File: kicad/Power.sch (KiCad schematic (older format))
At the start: 19 parts, among them U201 TPS54232, U202 TC1262-33

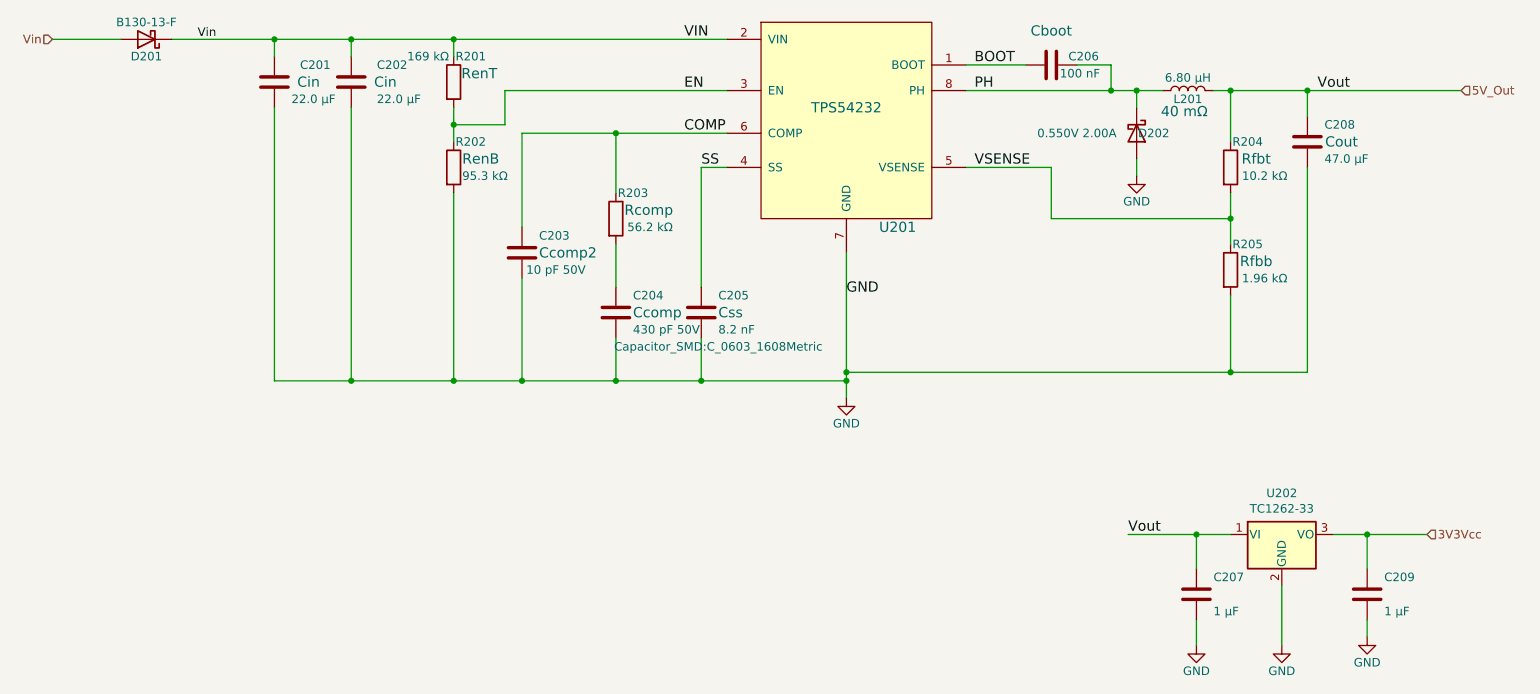
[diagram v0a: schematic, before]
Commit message: Updated the addresssing of the LCD
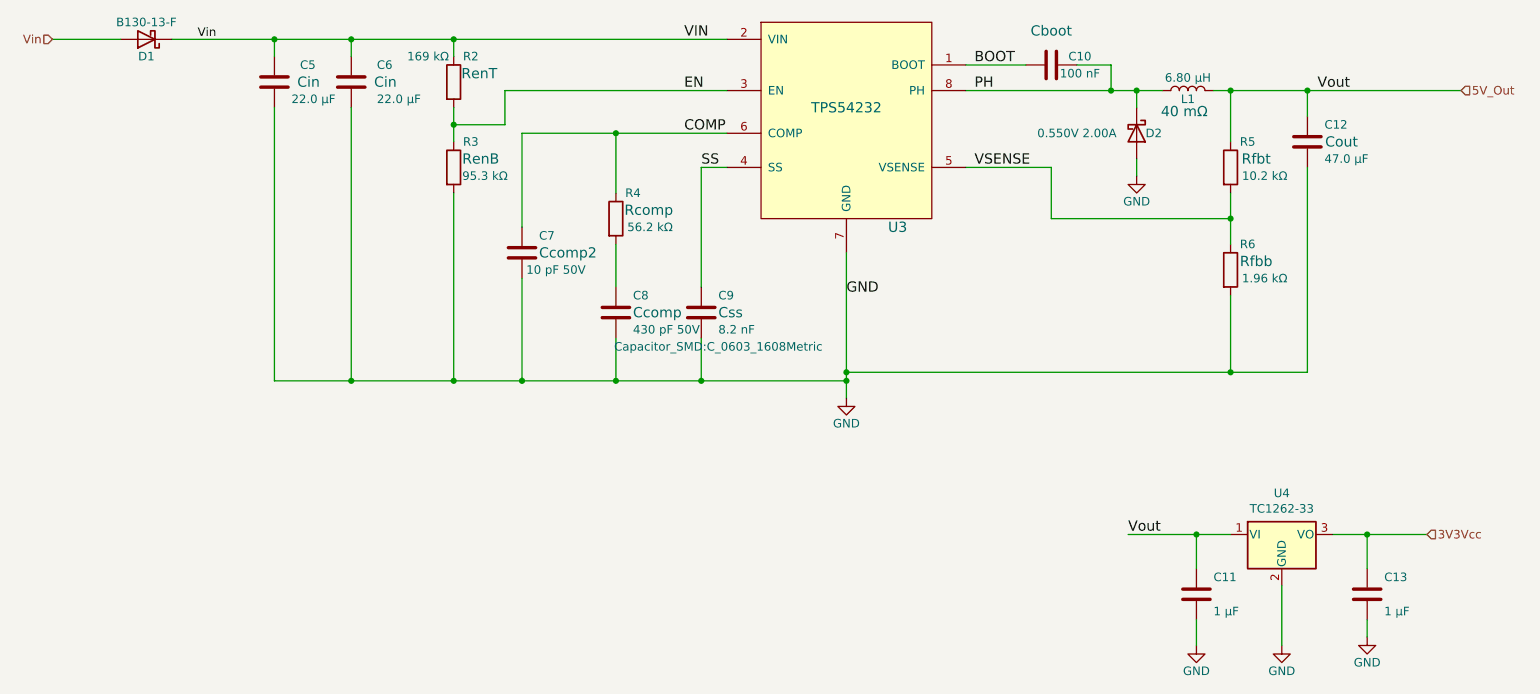
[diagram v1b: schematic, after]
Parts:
- renumbered C206 to C10, C207 to C11, C208 to C12, C209 to C13, C201 to C5, C202 to C6, C203 to C7, C204 to C8, C205 to C9, D201 to D1, D202 to D2, L201 to L1, R201 to R2, R202 to R3, R203 to R4, R204 to R5, R205 to R6, U201 to U3, U202 to U4
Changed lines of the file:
@@
 $EndDescr
 $Comp
-L FieldDevice_Power_5V-rescue:TPS54232-FieldDevice_Power_5V U201
+L FieldDevice_Power_5V-rescue:TPS54232-FieldDevice_Power_5V U3
 U 1 1 5A47974C
 P 5600 1700
-F 0 "U201" H 5900 1000 60  0000 C CNN
+F 0 "U3" H 5900 1000 60  0000 C CNN
 F 1 "TPS54232" H 5600 1700 60  0000 C CNN
 F 2 "FieldDevice_Power_5V:TPS54232DR" H 5600 1750 60  0001 C CNN
@@
 $EndComp
 $Comp
-L Device:R R201
+L Device:R R2
 U 1 1 5A47979B
 P 3300 1550
-F 0 "R201" H 3400 1700 50  0000 C CNN
+F 0 "R2" H 3400 1700 50  0000 C CNN
 F 1 "169 kΩ" H 3150 1700 50  0000 C CNN
 F 2 "Resistor_SMD:R_0805_2012Metric" V 3230 1550 50  0001 C CNN
@@
 $EndComp
 $Comp
-L Device:R R202
+L Device:R R3
 U 1 1 5A47981A
 P 3300 2050
-F 0 "R202" H 3400 2200 50  0000 C CNN
+F 0 "R3" H 3400 2200 50  0000 C CNN
 F 1 "95.3 kΩ" H 3350 2000 50  0000 L CNN
 F 2 "Resistor_SMD:R_0805_2012Metric" V 3230 2050 50  0001 C CNN
@@
 $EndComp
 $Comp
-L Device:R R203
+L Device:R R4
 U 1 1 5A47984F
 P 4250 2350
-F 0 "R203" H 4350 2500 50  0000 C CNN
+F 0 "R4" H 4350 2500 50  0000 C CNN
 F 1 "56.2 kΩ" H 4450 2300 50  0000 C CNN
 F 2 "Resistor_SMD:R_0805_2012Metric" V 4180 2350 50  0001 C CNN
@@
 $EndComp
 $Comp
-L Device:R R204
+L Device:R R5
 U 1 1 5A479895
 P 7850 2050
-F 0 "R204" H 7950 2200 50  0000 C CNN
+F 0 "R5" H 7950 2200 50  0000 C CNN
 F 1 "10.2 kΩ" H 8050 2000 50  0000 C CNN
 F 2 "Resistor_SMD:R_0805_2012Metric" V 7780 2050 50  0001 C CNN
@@
 $EndComp
 $Comp
-L Device:R R205
+L Device:R R6
 U 1 1 5A479906
 P 7850 2650
-F 0 "R205" H 7950 2800 50  0000 C CNN
+F 0 "R6" H 7950 2800 50  0000 C CNN
 F 1 "1.96 kΩ" H 8050 2600 50  0000 C CNN
 F 2 "Resistor_SMD:R_0805_2012Metric" V 7780 2650 50  0001 C CNN
@@
 $EndComp
 $Comp
-L Device:C C201
+L Device:C C5
 U 1 1 5A479940
 P 2250 1550
-F 0 "C201" H 2400 1650 50  0000 L CNN
+F 0 "C5" H 2400 1650 50  0000 L CNN
 F 1 "22.0 μF" H 2350 1450 50  0000 L CNN
 F 2 "Capacitor_SMD:C_1210_3225Metric" H 2100 1450 50  0001 C CNN
@@
 $EndComp
 $Comp
-L Device:C C203
+L Device:C C7
 U 1 1 5A4799E0
 P 3700 2550
-F 0 "C203" H 3800 2650 50  0000 L CNN
+F 0 "C7" H 3800 2650 50  0000 L CNN
 F 1 "10 pF 50V" H 3725 2450 50  0000 L CNN
 F 2 "Capacitor_SMD:C_0805_2012Metric" H 3738 2400 50  0001 C CNN
@@
 $EndComp
 $Comp
-L Device:C C204
+L Device:C C8
 U 1 1 5A479A24
 P 4250 2900
-F 0 "C204" H 4350 3000 50  0000 L CNN
+F 0 "C8" H 4350 3000 50  0000 L CNN
 F 1 "430 pF 50V" H 4350 2800 50  0000 L CNN
 F 2 "Capacitor_SMD:C_0805_2012Metric" H 4288 2750 50  0001 C CNN
@@
 $EndComp
 $Comp
-L Device:C C205
+L Device:C C9
 U 1 1 5A479A65
 P 4750 2900
-F 0 "C205" H 4850 3000 50  0000 L CNN
+F 0 "C9" H 4850 3000 50  0000 L CNN
 F 1 "8.2 nF" H 4850 2800 50  0000 L CNN
 F 2 "Capacitor_SMD:C_0603_1608Metric" H 4850 2700 50  0000 C CNN
@@
 $EndComp
 $Comp
-L Device:C C206
+L Device:C C10
 U 1 1 5A479AA7
 P 6800 1450
-F 0 "C206" V 6750 1550 50  0000 L CNN
+F 0 "C10" V 6750 1550 50  0000 L CNN
 F 1 "100 nF" V 6850 1500 50  0000 L CNN
 F 2 "Capacitor_SMD:C_0805_2012Metric" H 6838 1300 50  0001 C CNN
@@
 $EndComp
 $Comp
-L Device:C C208
+L Device:C C12
 U 1 1 5A479B0E
 P 8300 1900
-F 0 "C208" H 8400 2000 50  0000 L CNN
+F 0 "C12" H 8400 2000 50  0000 L CNN
 F 1 "47.0 μF" H 8400 1800 50  0000 L CNN
 F 2 "Capacitor_SMD:C_0805_2012Metric" H 8338 1750 50  0001 C CNN
@@
 $EndComp
 $Comp
-L Device:L L201
+L Device:L L1
 U 1 1 5A479B7A
 P 7600 1600
-F 0 "L201" V 7550 1600 50  0000 C CNN
+F 0 "L1" V 7550 1600 50  0000 C CNN
 F 1 "6.80 μΗ" V 7675 1600 50  0000 C CNN
 F 2 "FieldDevice_Power_5V:SDR0805-6R8ML" H 7600 1600 50  0001 C CNN
@@
 $EndComp
 $Comp
-L Device:D_Schottky D202
+L Device:D_Schottky D2
 U 1 1 5A479CF1
 P 7300 1850
-F 0 "D202" V 7300 1950 50  0000 C CNN
+F 0 "D2" V 7300 1950 50  0000 C CNN
 F 1 "0.550V 2.00A" V 7300 1500 50  0000 C CNN
 F 2 "FieldDevice_Power_5V:D_SOD-123F" H 7300 1850 50  0001 C CNN
@@
 $EndComp
 $Comp
-L Device:C C202
+L Device:C C6
 U 1 1 5A47A146
 P 2700 1550
-F 0 "C202" H 2850 1650 50  0000 L CNN
+F 0 "C6" H 2850 1650 50  0000 L CNN
 F 1 "22.0 μF" H 2850 1450 50  0000 L CNN
 F 2 "Capacitor_SMD:C_1210_3225Metric" H 2600 1650 50  0001 C CNN
@@
 	3300 1700 3300 1800
 $Comp
-L power:GND #PWR0201
+L power:GND #PWR011
 U 1 1 5A47B13B
 P 5600 3400
-F 0 "#PWR0201" H 5600 3150 50  0001 C CNN
+F 0 "#PWR011" H 5600 3150 50  0001 C CNN
 F 1 "GND" H 5600 3250 50  0000 C CNN
 F 2 "" H 5600 3400 50  0001 C CNN
@@
 $EndComp
 $Comp
-L power:GND #PWR0202
+L power:GND #PWR012
 U 1 1 5A47B17A
 P 7300 2100
-F 0 "#PWR0202" H 7300 1850 50  0001 C CNN
+F 0 "#PWR012" H 7300 1850 50  0001 C CNN
 F 1 "GND" H 7300 1950 50  0000 C CNN
 F 2 "" H 7300 2100 50  0001 C CNN
@@
 Vout
 $Comp
-L Device:D_Schottky D201
+L Device:D_Schottky D1
 U 1 1 5A482394
 P 1500 1300
-F 0 "D201" H 1500 1400 50  0000 C CNN
+F 0 "D1" H 1500 1400 50  0000 C CNN
 F 1 "B130-13-F" H 1500 1200 50  0000 C CNN
 F 2 "FieldDevice_Power_5V:B130-13-F" H 1500 1300 50  0001 C CNN
@@
 5V_Out
 $Comp
-L Regulator_Linear:TC1262-33 U202
+L Regulator_Linear:TC1262-33 U4
 U 1 1 5F29C039
 P 8150 4200
-F 0 "U202" H 8150 4442 50  0000 C CNN
+F 0 "U4" H 8150 4442 50  0000 C CNN
 F 1 "TC1262-33" H 8150 4351 50  0000 C CNN
 F 2 "" H 8150 4425 50  0001 C CIN
@@
 	8150 4500 8150 4850
 $Comp
-L power:GND #PWR0204
+L power:GND #PWR014
 U 1 1 5F2AC1B9
 P 8150 4850
-F 0 "#PWR0204" H 8150 4600 50  0001 C CNN
+F 0 "#PWR014" H 8150 4600 50  0001 C CNN
 F 1 "GND" H 8150 4700 50  0000 C CNN
 F 2 "" H 8150 4850 50  0001 C CNN
@@
 $EndComp
 $Comp
-L Device:C C207
+L Device:C C11
 U 1 1 5F2ACA63
 P 7650 4550
-F 0 "C207" H 7750 4650 50  0000 L CNN
+F 0 "C11" H 7750 4650 50  0000 L CNN
 F 1 "1 μF" H 7750 4450 50  0000 L CNN
 F 2 "Capacitor_SMD:C_0805_2012Metric" H 7688 4400 50  0001 C CNN
@@
 	8650 4200 9000 4200
 $Comp
-L power:GND #PWR0203
+L power:GND #PWR013
 U 1 1 5F2AE872
 P 7650 4850
-F 0 "#PWR0203" H 7650 4600 50  0001 C CNN
+F 0 "#PWR013" H 7650 4600 50  0001 C CNN
 F 1 "GND" H 7650 4700 50  0000 C CNN
 F 2 "" H 7650 4850 50  0001 C CNN
@@
 	7650 4200 7250 4200
 $Comp
-L Device:C C209
+L Device:C C13
 U 1 1 5F2B414B
 P 8650 4550
-F 0 "C209" H 8750 4650 50  0000 L CNN
+F 0 "C13" H 8750 4650 50  0000 L CNN
 F 1 "1 μF" H 8750 4450 50  0000 L CNN
 F 2 "Capacitor_SMD:C_0805_2012Metric" H 8688 4400 50  0001 C CNN
@@
 $EndComp
 $Comp
-L power:GND #PWR0205
+L power:GND #PWR015
 U 1 1 5F2B4985
 P 8650 4800
-F 0 "#PWR0205" H 8650 4550 50  0001 C CNN
+F 0 "#PWR015" H 8650 4550 50  0001 C CNN
 F 1 "GND" H 8650 4650 50  0000 C CNN
 F 2 "" H 8650 4800 50  0001 C CNN

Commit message: Updates the RC selection for the switch debounce
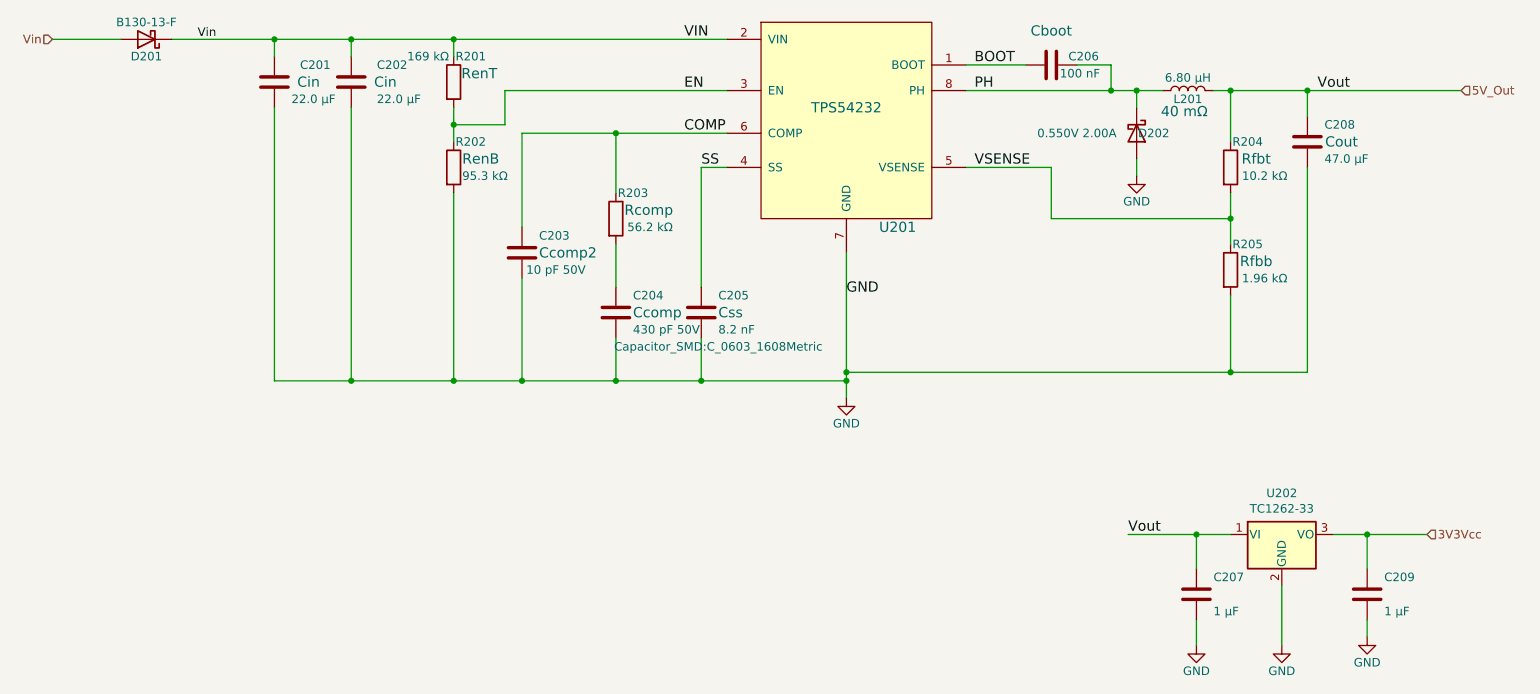
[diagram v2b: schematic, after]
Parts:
- renumbered C5 to C201, C6 to C202, C7 to C203, C8 to C204, C9 to C205, C10 to C206, C11 to C207, C12 to C208, C13 to C209, D1 to D201, D2 to D202, L1 to L201, R2 to R201, R3 to R202, R4 to R203, R5 to R204, R6 to R205, U3 to U201, U4 to U202
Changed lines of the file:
@@
 $EndDescr
 $Comp
-L FieldDevice_Power_5V-rescue:TPS54232-FieldDevice_Power_5V U3
+L FieldDevice_Power_5V-rescue:TPS54232-FieldDevice_Power_5V U201
 U 1 1 5A47974C
 P 5600 1700
-F 0 "U3" H 5900 1000 60  0000 C CNN
+F 0 "U201" H 5900 1000 60  0000 C CNN
 F 1 "TPS54232" H 5600 1700 60  0000 C CNN
 F 2 "FieldDevice_Power_5V:TPS54232DR" H 5600 1750 60  0001 C CNN
@@
 $EndComp
 $Comp
-L Device:R R2
+L Device:R R201
 U 1 1 5A47979B
 P 3300 1550
-F 0 "R2" H 3400 1700 50  0000 C CNN
+F 0 "R201" H 3400 1700 50  0000 C CNN
 F 1 "169 kΩ" H 3150 1700 50  0000 C CNN
 F 2 "Resistor_SMD:R_0805_2012Metric" V 3230 1550 50  0001 C CNN
@@
 $EndComp
 $Comp
-L Device:R R3
+L Device:R R202
 U 1 1 5A47981A
 P 3300 2050
-F 0 "R3" H 3400 2200 50  0000 C CNN
+F 0 "R202" H 3400 2200 50  0000 C CNN
 F 1 "95.3 kΩ" H 3350 2000 50  0000 L CNN
 F 2 "Resistor_SMD:R_0805_2012Metric" V 3230 2050 50  0001 C CNN
@@
 $EndComp
 $Comp
-L Device:R R4
+L Device:R R203
 U 1 1 5A47984F
 P 4250 2350
-F 0 "R4" H 4350 2500 50  0000 C CNN
+F 0 "R203" H 4350 2500 50  0000 C CNN
 F 1 "56.2 kΩ" H 4450 2300 50  0000 C CNN
 F 2 "Resistor_SMD:R_0805_2012Metric" V 4180 2350 50  0001 C CNN
@@
 $EndComp
 $Comp
-L Device:R R5
+L Device:R R204
 U 1 1 5A479895
 P 7850 2050
-F 0 "R5" H 7950 2200 50  0000 C CNN
+F 0 "R204" H 7950 2200 50  0000 C CNN
 F 1 "10.2 kΩ" H 8050 2000 50  0000 C CNN
 F 2 "Resistor_SMD:R_0805_2012Metric" V 7780 2050 50  0001 C CNN
@@
 $EndComp
 $Comp
-L Device:R R6
+L Device:R R205
 U 1 1 5A479906
 P 7850 2650
-F 0 "R6" H 7950 2800 50  0000 C CNN
+F 0 "R205" H 7950 2800 50  0000 C CNN
 F 1 "1.96 kΩ" H 8050 2600 50  0000 C CNN
 F 2 "Resistor_SMD:R_0805_2012Metric" V 7780 2650 50  0001 C CNN
@@
 $EndComp
 $Comp
-L Device:C C5
+L Device:C C201
 U 1 1 5A479940
 P 2250 1550
-F 0 "C5" H 2400 1650 50  0000 L CNN
+F 0 "C201" H 2400 1650 50  0000 L CNN
 F 1 "22.0 μF" H 2350 1450 50  0000 L CNN
 F 2 "Capacitor_SMD:C_1210_3225Metric" H 2100 1450 50  0001 C CNN
@@
 $EndComp
 $Comp
-L Device:C C7
+L Device:C C203
 U 1 1 5A4799E0
 P 3700 2550
-F 0 "C7" H 3800 2650 50  0000 L CNN
+F 0 "C203" H 3800 2650 50  0000 L CNN
 F 1 "10 pF 50V" H 3725 2450 50  0000 L CNN
 F 2 "Capacitor_SMD:C_0805_2012Metric" H 3738 2400 50  0001 C CNN
@@
 $EndComp
 $Comp
-L Device:C C8
+L Device:C C204
 U 1 1 5A479A24
 P 4250 2900
-F 0 "C8" H 4350 3000 50  0000 L CNN
+F 0 "C204" H 4350 3000 50  0000 L CNN
 F 1 "430 pF 50V" H 4350 2800 50  0000 L CNN
 F 2 "Capacitor_SMD:C_0805_2012Metric" H 4288 2750 50  0001 C CNN
@@
 $EndComp
 $Comp
-L Device:C C9
+L Device:C C205
 U 1 1 5A479A65
 P 4750 2900
-F 0 "C9" H 4850 3000 50  0000 L CNN
+F 0 "C205" H 4850 3000 50  0000 L CNN
 F 1 "8.2 nF" H 4850 2800 50  0000 L CNN
 F 2 "Capacitor_SMD:C_0603_1608Metric" H 4850 2700 50  0000 C CNN
@@
 $EndComp
 $Comp
-L Device:C C10
+L Device:C C206
 U 1 1 5A479AA7
 P 6800 1450
-F 0 "C10" V 6750 1550 50  0000 L CNN
+F 0 "C206" V 6750 1550 50  0000 L CNN
 F 1 "100 nF" V 6850 1500 50  0000 L CNN
 F 2 "Capacitor_SMD:C_0805_2012Metric" H 6838 1300 50  0001 C CNN
@@
 $EndComp
 $Comp
-L Device:C C12
+L Device:C C208
 U 1 1 5A479B0E
 P 8300 1900
-F 0 "C12" H 8400 2000 50  0000 L CNN
+F 0 "C208" H 8400 2000 50  0000 L CNN
 F 1 "47.0 μF" H 8400 1800 50  0000 L CNN
 F 2 "Capacitor_SMD:C_0805_2012Metric" H 8338 1750 50  0001 C CNN
@@
 $EndComp
 $Comp
-L Device:L L1
+L Device:L L201
 U 1 1 5A479B7A
 P 7600 1600
-F 0 "L1" V 7550 1600 50  0000 C CNN
+F 0 "L201" V 7550 1600 50  0000 C CNN
 F 1 "6.80 μΗ" V 7675 1600 50  0000 C CNN
 F 2 "FieldDevice_Power_5V:SDR0805-6R8ML" H 7600 1600 50  0001 C CNN
@@
 $EndComp
 $Comp
-L Device:D_Schottky D2
+L Device:D_Schottky D202
 U 1 1 5A479CF1
 P 7300 1850
-F 0 "D2" V 7300 1950 50  0000 C CNN
+F 0 "D202" V 7300 1950 50  0000 C CNN
 F 1 "0.550V 2.00A" V 7300 1500 50  0000 C CNN
 F 2 "FieldDevice_Power_5V:D_SOD-123F" H 7300 1850 50  0001 C CNN
@@
 $EndComp
 $Comp
-L Device:C C6
+L Device:C C202
 U 1 1 5A47A146
 P 2700 1550
-F 0 "C6" H 2850 1650 50  0000 L CNN
+F 0 "C202" H 2850 1650 50  0000 L CNN
 F 1 "22.0 μF" H 2850 1450 50  0000 L CNN
 F 2 "Capacitor_SMD:C_1210_3225Metric" H 2600 1650 50  0001 C CNN
@@
 	3300 1700 3300 1800
 $Comp
-L power:GND #PWR011
+L power:GND #PWR0201
 U 1 1 5A47B13B
 P 5600 3400
-F 0 "#PWR011" H 5600 3150 50  0001 C CNN
+F 0 "#PWR0201" H 5600 3150 50  0001 C CNN
 F 1 "GND" H 5600 3250 50  0000 C CNN
 F 2 "" H 5600 3400 50  0001 C CNN
@@
 $EndComp
 $Comp
-L power:GND #PWR012
+L power:GND #PWR0202
 U 1 1 5A47B17A
 P 7300 2100
-F 0 "#PWR012" H 7300 1850 50  0001 C CNN
+F 0 "#PWR0202" H 7300 1850 50  0001 C CNN
 F 1 "GND" H 7300 1950 50  0000 C CNN
 F 2 "" H 7300 2100 50  0001 C CNN
@@
 Vout
 $Comp
-L Device:D_Schottky D1
+L Device:D_Schottky D201
 U 1 1 5A482394
 P 1500 1300
-F 0 "D1" H 1500 1400 50  0000 C CNN
+F 0 "D201" H 1500 1400 50  0000 C CNN
 F 1 "B130-13-F" H 1500 1200 50  0000 C CNN
 F 2 "FieldDevice_Power_5V:B130-13-F" H 1500 1300 50  0001 C CNN
@@
 5V_Out
 $Comp
-L Regulator_Linear:TC1262-33 U4
+L Regulator_Linear:TC1262-33 U202
 U 1 1 5F29C039
 P 8150 4200
-F 0 "U4" H 8150 4442 50  0000 C CNN
+F 0 "U202" H 8150 4442 50  0000 C CNN
 F 1 "TC1262-33" H 8150 4351 50  0000 C CNN
 F 2 "" H 8150 4425 50  0001 C CIN
@@
 	8150 4500 8150 4850
 $Comp
-L power:GND #PWR014
+L power:GND #PWR0204
 U 1 1 5F2AC1B9
 P 8150 4850
-F 0 "#PWR014" H 8150 4600 50  0001 C CNN
+F 0 "#PWR0204" H 8150 4600 50  0001 C CNN
 F 1 "GND" H 8150 4700 50  0000 C CNN
 F 2 "" H 8150 4850 50  0001 C CNN
@@
 $EndComp
 $Comp
-L Device:C C11
+L Device:C C207
 U 1 1 5F2ACA63
 P 7650 4550
-F 0 "C11" H 7750 4650 50  0000 L CNN
+F 0 "C207" H 7750 4650 50  0000 L CNN
 F 1 "1 μF" H 7750 4450 50  0000 L CNN
 F 2 "Capacitor_SMD:C_0805_2012Metric" H 7688 4400 50  0001 C CNN
@@
 	8650 4200 9000 4200
 $Comp
-L power:GND #PWR013
+L power:GND #PWR0203
 U 1 1 5F2AE872
 P 7650 4850
-F 0 "#PWR013" H 7650 4600 50  0001 C CNN
+F 0 "#PWR0203" H 7650 4600 50  0001 C CNN
 F 1 "GND" H 7650 4700 50  0000 C CNN
 F 2 "" H 7650 4850 50  0001 C CNN
@@
 	7650 4200 7250 4200
 $Comp
-L Device:C C13
+L Device:C C209
 U 1 1 5F2B414B
 P 8650 4550
-F 0 "C13" H 8750 4650 50  0000 L CNN
+F 0 "C209" H 8750 4650 50  0000 L CNN
 F 1 "1 μF" H 8750 4450 50  0000 L CNN
 F 2 "Capacitor_SMD:C_0805_2012Metric" H 8688 4400 50  0001 C CNN
@@
 $EndComp
 $Comp
-L power:GND #PWR015
+L power:GND #PWR0205
 U 1 1 5F2B4985
 P 8650 4800
-F 0 "#PWR015" H 8650 4550 50  0001 C CNN
+F 0 "#PWR0205" H 8650 4550 50  0001 C CNN
 F 1 "GND" H 8650 4650 50  0000 C CNN
 F 2 "" H 8650 4800 50  0001 C CNN
